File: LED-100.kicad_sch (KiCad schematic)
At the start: 101 parts, among them J2 LDA100_2_J2, J3 LDA100_2_J3, J4 LDA100_2_J4, J5 xtra, J7 Conn_01x01, J8 Conn_01x07, SW1 SW_SPDT, SW2 SW_SPST, U1 TLC5947DAP, U2 TLC5947DAP, U3 TLC5947DAP, U4 TEENSY 4.0

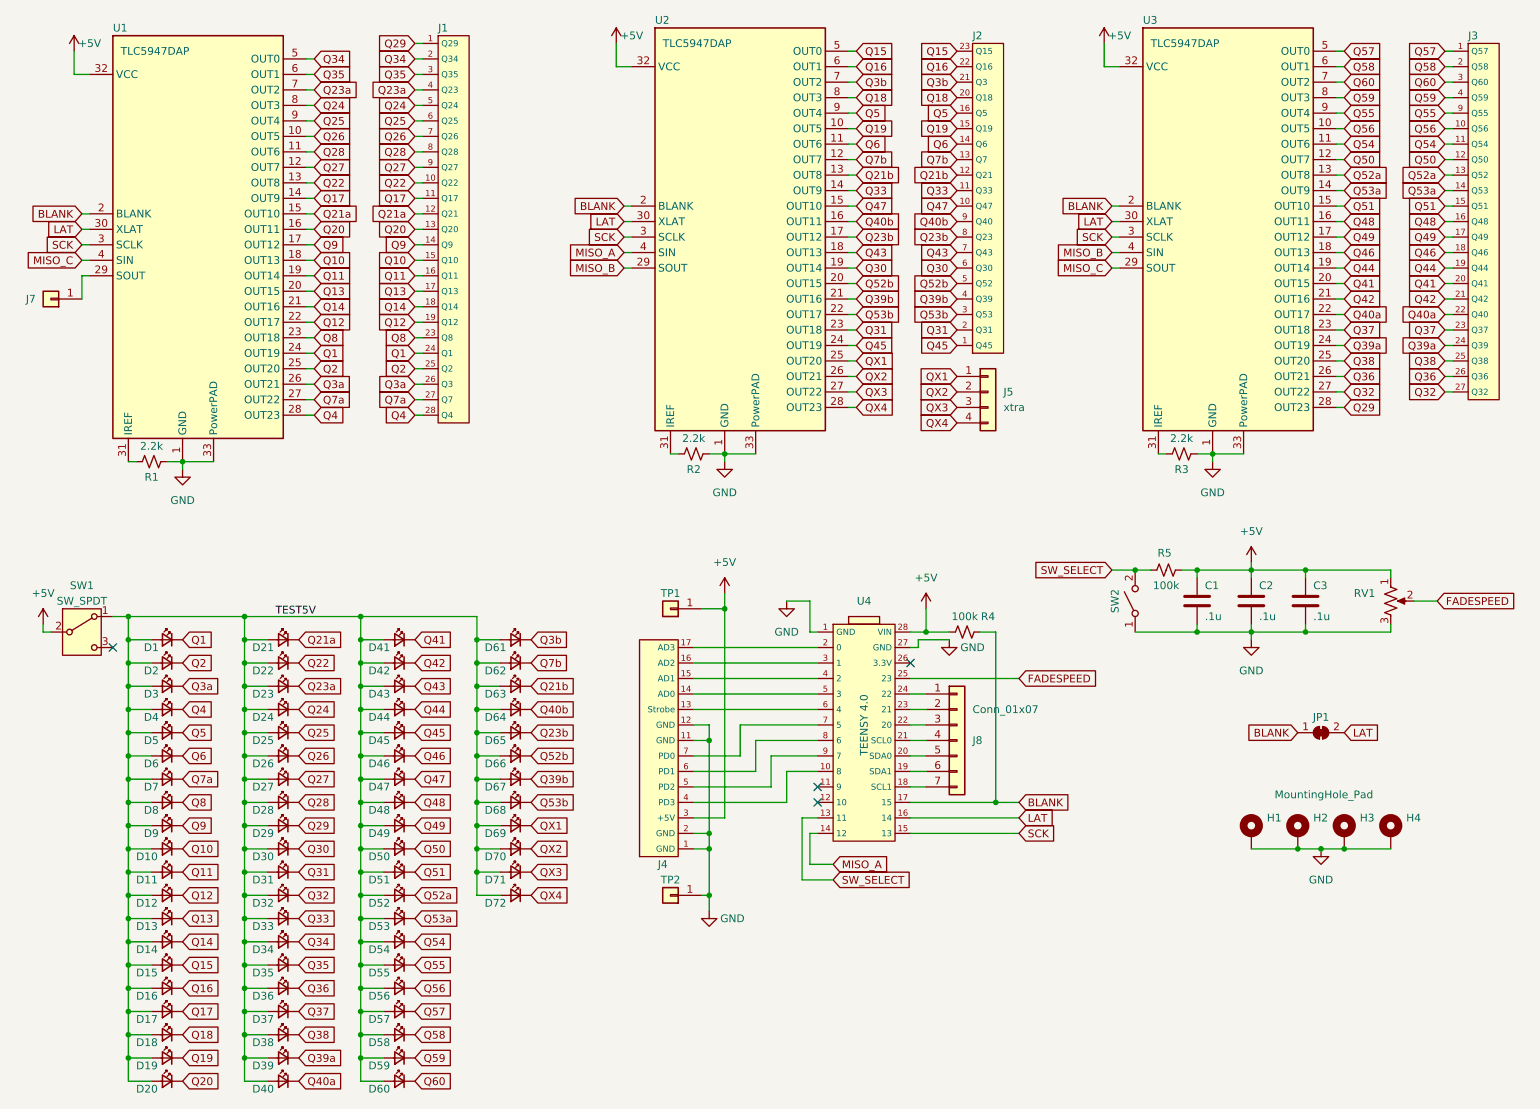
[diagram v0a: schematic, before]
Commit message: <---wider--->
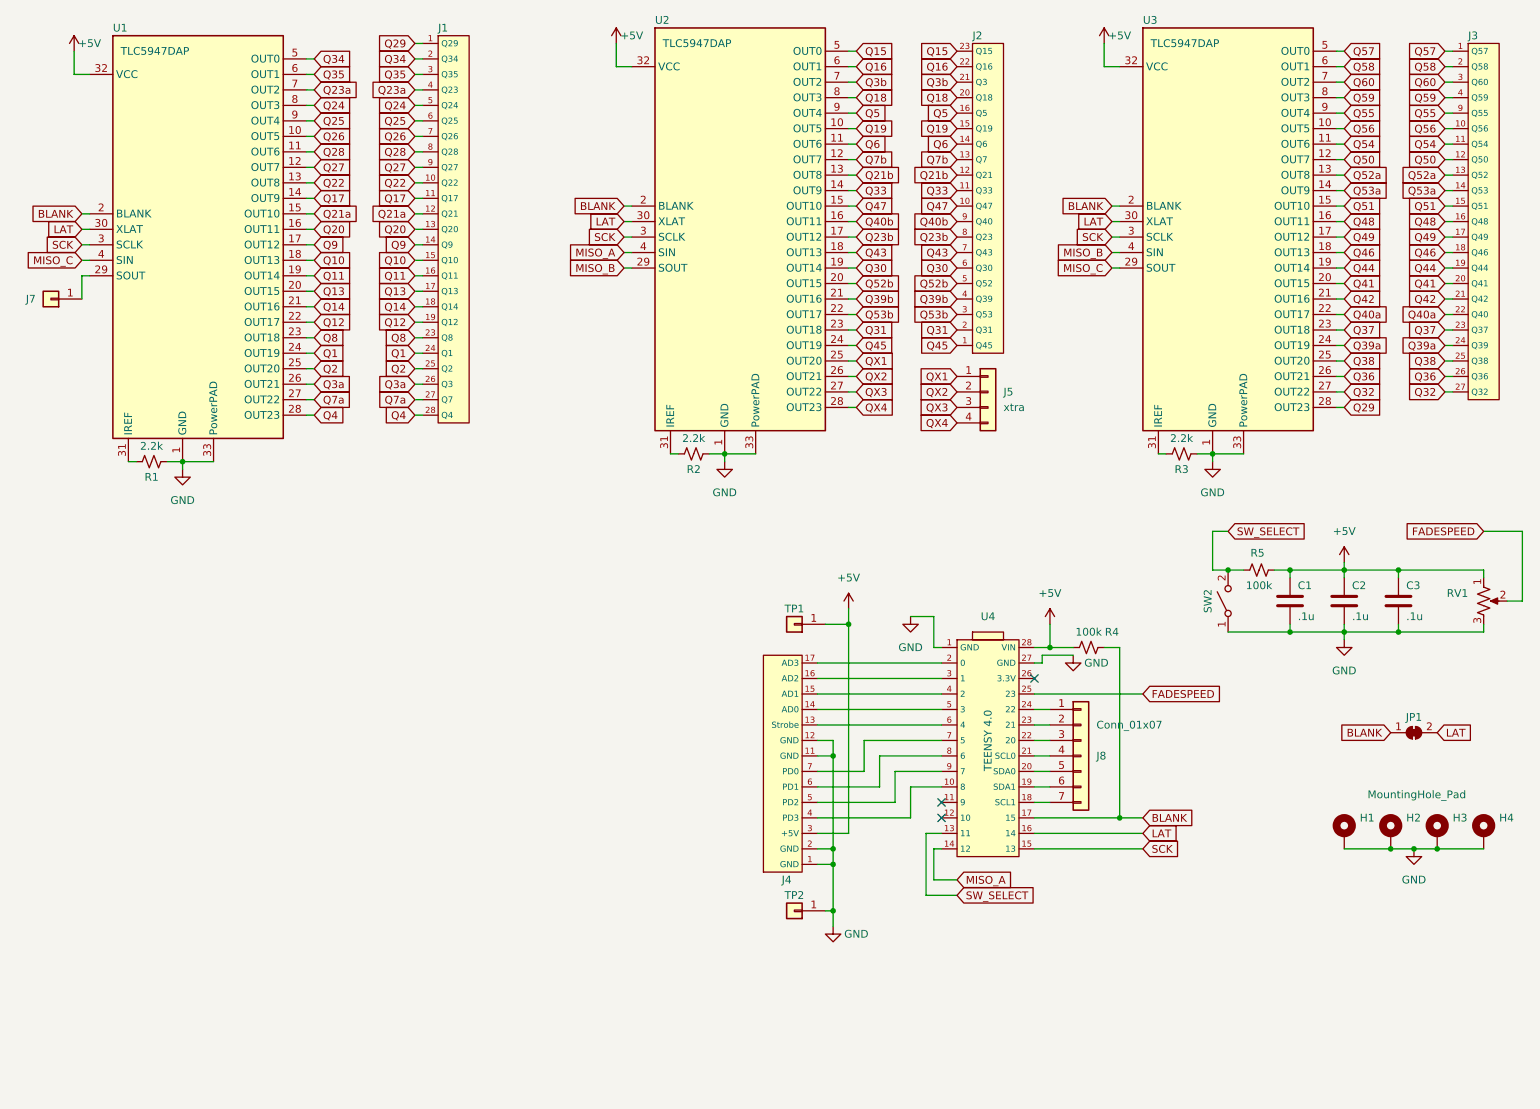
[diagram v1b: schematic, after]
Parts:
- removed D1, D10, D11, D12, D13, D14, D15, D16, D17, D18, D19, D2, D20, D21, D22, D23, D24, D25, D26, D27, D28, D29, D3, D30, D31, D32, D33, D34, D35, D36, D37, D38, D39, D4, D40, D41, D42, D43, D44, D45, D46, D47, D48, D49, D5, D50, D51, D52, D53, D54, D55, D56, D57, D58, D59, D6, D60, D61, D62, D63, D64, D65, D66, D67, D68, D69, D7, D70, D71, D72, D8, D9: LED_Small, LED_THT:LED_D3.0mm, symbol Device:LED_Small
- removed SW1: SW_SPDT, MyParts:SWITCH_SPDT-SLW-12689-4A-N-D, symbol Switch:SW_SPDT
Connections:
- no-connect marks 4 -> 3
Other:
- moved on the sheet: C1, C2, C3, H1, H2, H3, H4, J4, J8, JP1, R4, R5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
